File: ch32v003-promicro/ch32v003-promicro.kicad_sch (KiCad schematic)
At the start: 21 parts, among them J1 USB2.0_C_v3, J2 ProMicro-LeftPin, J3 ProMicro-RightPin, SW1 SW_Push, U1 CH32V003F4P6, U2 AMS1117-3.3, Y1 24M

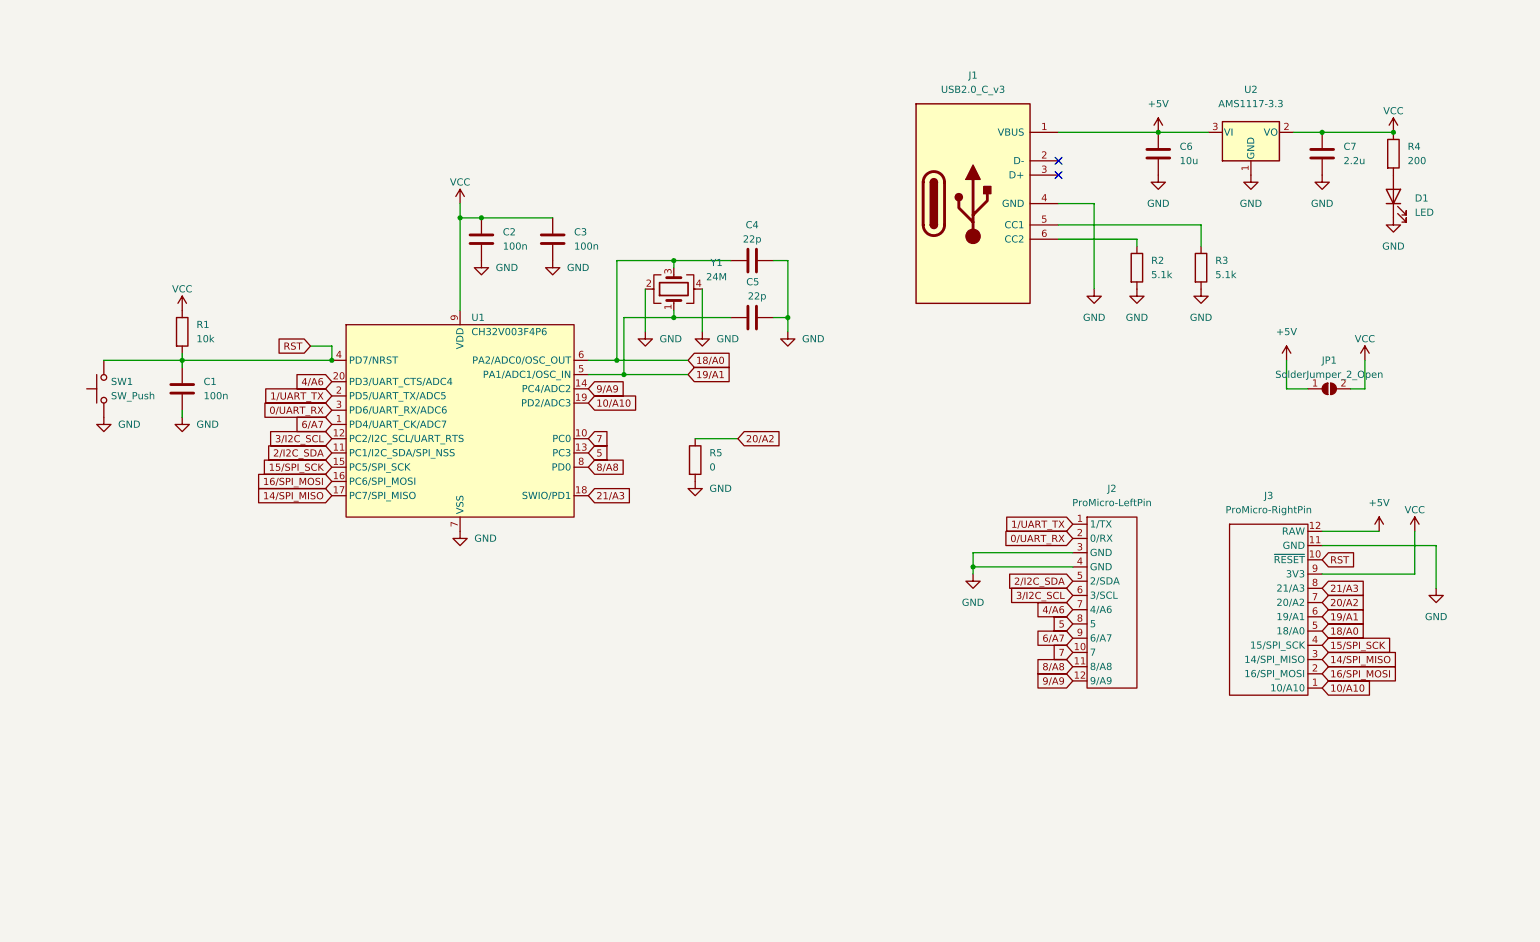
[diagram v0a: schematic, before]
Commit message: ch32v003promicro/1.1.0
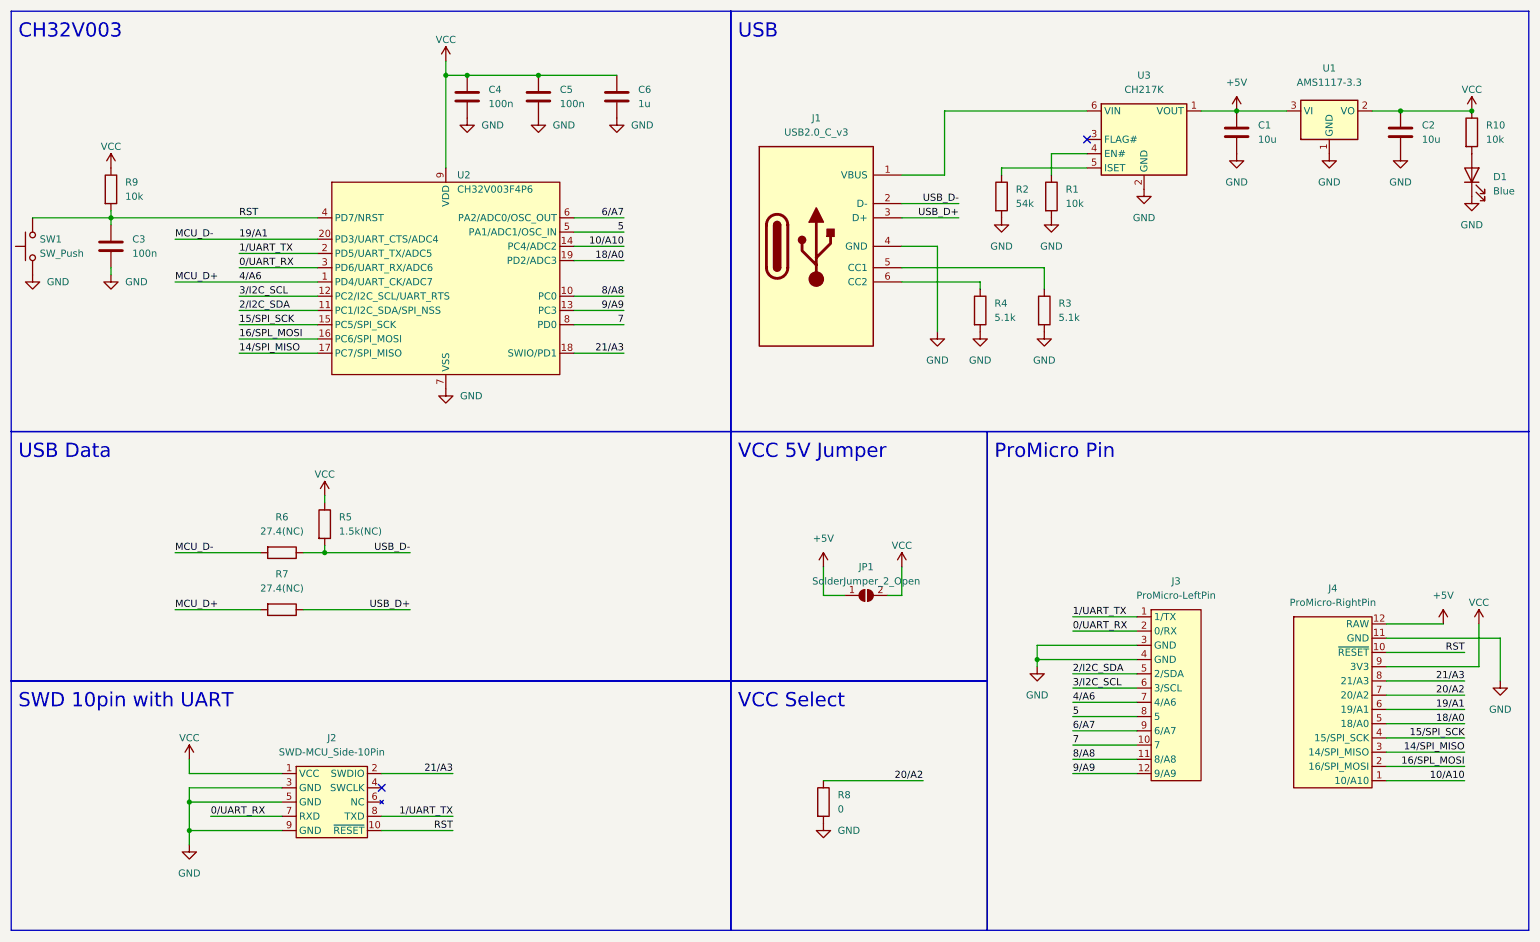
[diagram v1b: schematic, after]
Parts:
- removed C4, C5: 22p, $74th:Capacitor_0805_2012, symbol Device:C
- removed Y1: 24M, $74th:Crystal_SMD_3225-4Pin_3.2x2.5mm_HandSoldering, symbol Device:Crystal_GND24
- added C6: 1u, $74th:Capacitor_0805_2012, symbol Device:C
- added J2: SWD-MCU_Side-10Pin, $74th:SWD_2x05_P1.27mm, symbol $74th:SWD-MCU_Side-10Pin
- added R1: 10k, $74th:Register_0805_2012, symbol Device:R
- added R2: 54k, $74th:Register_0805_2012, symbol Device:R
- added R5: 1.5k(NC), $74th:Register_0805_2012, symbol Device:R
- added R6, R7: 27.4(NC), $74th:Register_0805_2012, symbol Device:R
- added U3: CH217K, Package_TO_SOT_SMD:SOT-23-6, symbol $74th:CH217K-USB_Power_Limit_Switch
- C2: renamed from C7; value 2.2u -> 10u
- D1: value LED -> Blue
- R10: renamed from R4; value 200 -> 10k
- renumbered C6 to C1, C1 to C3, C2 to C4, C3 to C5, J2 to J3, J3 to J4, R2 to R4, R5 to R8, R1 to R9, U2 to U1, U1 to U2
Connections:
- net +5V: now also U3.1 (VOUT); no longer J1.1 (VBUS)
- net 0/UART_RX: now also J2.7 (RXD)
- net 10/A10: now also U2.14 (PC4/ADC2); no longer U2.19 (PD2/ADC3)
- net 18/A0: now also U2.19 (PD2/ADC3); no longer U2.6 (PA2/ADC0/OSC_OUT)
- net 19/A1: now also U2.20 (PD3/UART_CTS/ADC4), R6.2; no longer U2.5 (PA1/ADC1/OSC_IN)
- net 1/UART_TX: now also J2.8 (TXD)
- net 21/A3: now also J2.2 (SWDIO)
- net 4/A6: now also U2.1 (PD4/UART_CK/ADC7), R7.2; no longer U2.20 (PD3/UART_CTS/ADC4)
- net 5: now also U2.5 (PA1/ADC1/OSC_IN); no longer U2.13 (PC3)
- net 6/A7: now also U2.6 (PA2/ADC0/OSC_OUT); no longer U2.1 (PD4/UART_CK/ADC7)
- net 7: now also U2.8 (PD0); no longer U2.10 (PC0)
- net 8/A8: now also U2.10 (PC0); no longer U2.8 (PD0)
- net 9/A9: now also U2.13 (PC3); no longer U2.14 (PC4/ADC2)
- net GND: now also C6.2, J2.3 (GND), J2.5 (GND), J2.9 (GND), R1.2, R2.2, U3.2 (GND)
- net RST: now also J2.10 (~{RESET})
- net VCC: now also C6.1, J2.1 (VCC), R5.1
- net USB_D-: now reaches J1.2 (D-)
- net USB_D-: now also R5.2, R6.1
- net USB_D+: now reaches J1.3 (D+)
- net USB_D+: now also R7.1
- net 16/SPI_MOSI renamed 16/SPL_MOSI
- new net: R1.1, U3.4 (EN#)
- new net: J1.1 (VBUS), U3.6 (VIN)
- new net: R2.1, U3.5 (ISET)
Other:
- note added: "CH32V003"
- note added: "ProMicro Pin"
- note added: "SWD 10pin with UART"
- note added: "USB"
- note added: "USB Data"
- note added: "VCC 5V Jumper"
- note added: "VCC Select"
- moved on the sheet: C1, C2, C3, C4, C5, D1, J1, JP1, R10, R3, R4, R8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
